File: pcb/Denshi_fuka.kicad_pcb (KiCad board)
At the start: 2 copper layers, 68.6 x 53.3 mm, 8 parts, among them J1 Power, J2 Digital/PWM, J3 Analog, J4 Digital/PWM

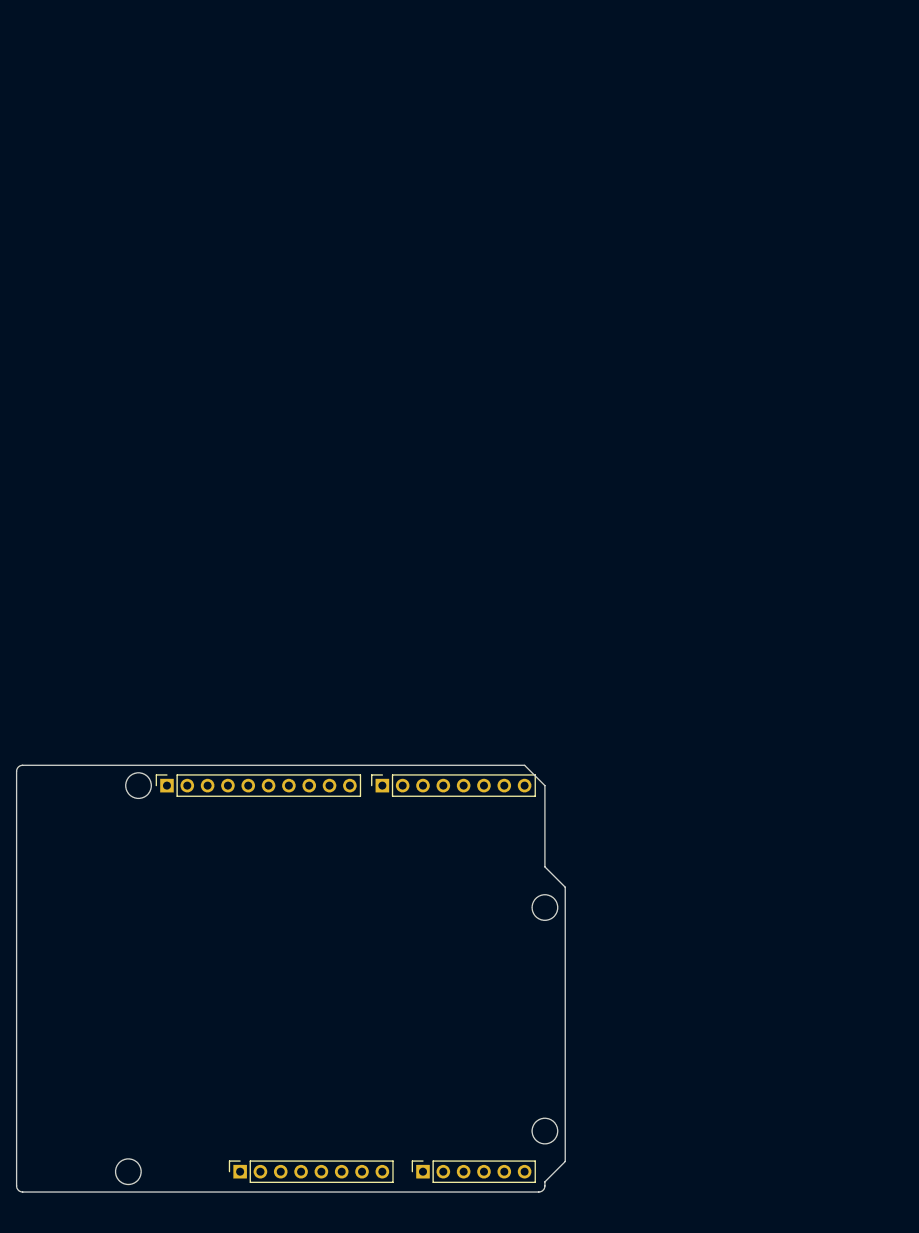
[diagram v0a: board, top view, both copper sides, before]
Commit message: Fuck
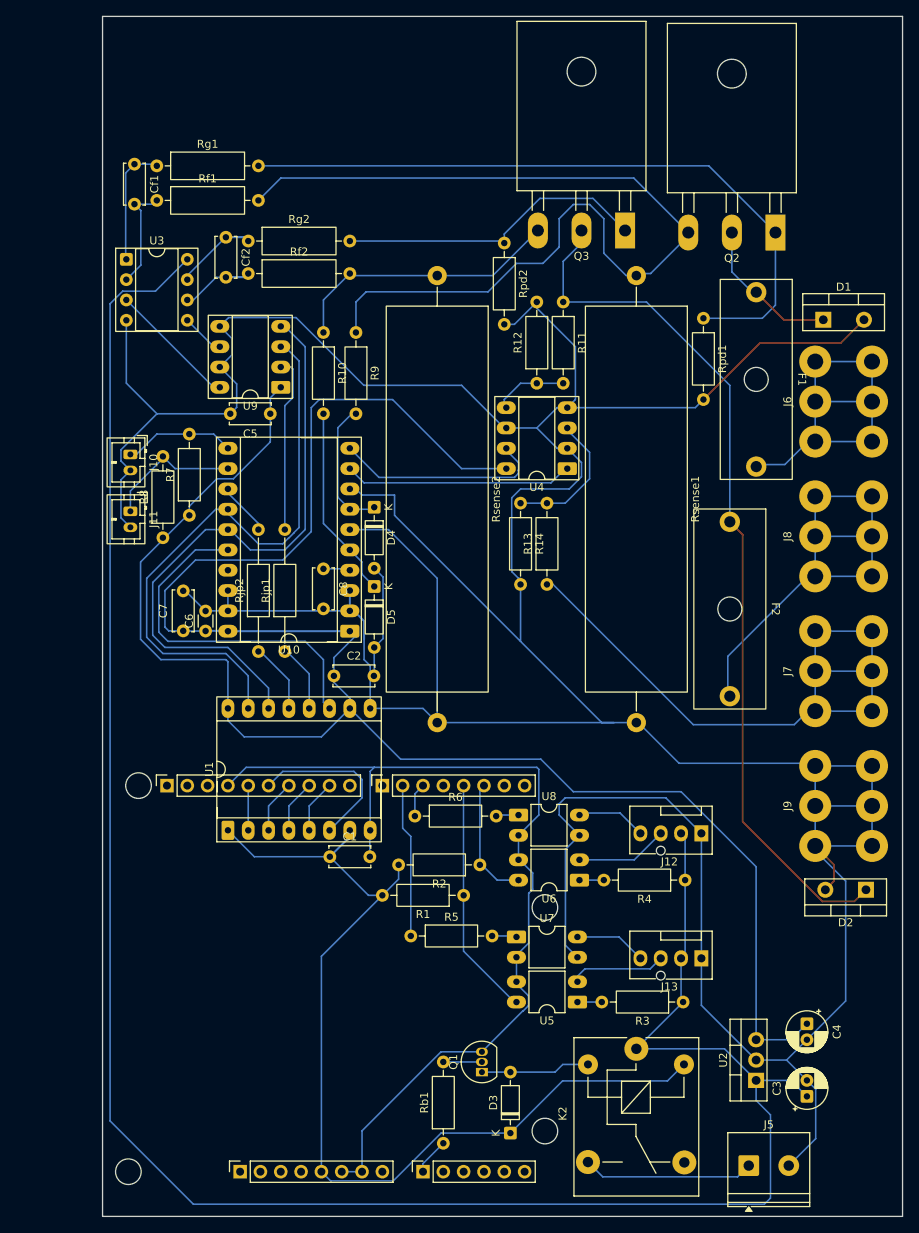
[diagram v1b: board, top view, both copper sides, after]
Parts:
- added C1: 0.1uF, Capacitor_THT:C_Disc_D5.0mm_W2.5mm_P5.00mm, F.Cu at (139.2, 58.1)
- added C2: 0.1uF, Capacitor_THT:C_Disc_D5.0mm_W2.5mm_P5.00mm, F.Cu at (139.7, 35.5)
- added C3: 10uF, Capacitor_THT:CP_Radial_D5.0mm_P2.00mm, F.Cu at (198.8, 88.0)
- added C4: 10uF, Capacitor_THT:CP_Radial_D5.0mm_P2.00mm, F.Cu at (198.8, 79.0)
- added C5: 0.1uF, Capacitor_THT:C_Disc_D5.0mm_W2.5mm_P5.00mm, F.Cu at (131.7, 2.72)
- added C6: 1uF, Capacitor_THT:C_Disc_D3.0mm_W1.6mm_P2.50mm, F.Cu at (123.6, 29.9)
- added C7: 0.1uF, Capacitor_THT:C_Disc_D5.0mm_W2.5mm_P5.00mm, F.Cu at (120.8, 29.9)
- added C8: 0.1uF, Capacitor_THT:C_Disc_D5.0mm_W2.5mm_P5.00mm, F.Cu at (138.4, 22.1)
- added Cf1: 0.1uF, Capacitor_THT:C_Disc_D5.0mm_W2.5mm_P5.00mm, F.Cu at (114.7, -28.5)
- added Cf2: 0.1uF, Capacitor_THT:C_Disc_D5.0mm_W2.5mm_P5.00mm, F.Cu at (126.2, -19.3)
- added D1: D, Package_TO_SOT_THT:TO-220-2_Vertical, F.Cu at (200.8, -9.03)
- added D2: D, Package_TO_SOT_THT:TO-220-2_Vertical, F.Cu at (206.2, 62.2)
- added D3: 1N4148, Diode_THT:D_DO-35_SOD27_P7.62mm_Horizontal, F.Cu at (161.7, 92.6)
- added D4: D_Zener_3V3, Diode_THT:D_DO-35_SOD27_P7.62mm_Horizontal, F.Cu at (144.7, 14.4)
- added D5: D_Zener_3V3, Diode_THT:D_DO-35_SOD27_P7.62mm_Horizontal, F.Cu at (144.7, 24.3)
- added F1: Fuse, MyParts:MF-563, F.Cu at (192.5, -1.58)
- added F2: Fuse, MyParts:MF-563, F.Cu at (189.2, 27.1)
- added J10: JST_PH2P, Connector_JST:JST_PH_B2B-PH-K_1x02_P2.00mm_Vertical, F.Cu at (114.2, 7.80)
- added J11: JST_PH2P, Connector_JST:JST_PH_B2B-PH-K_1x02_P2.00mm_Vertical, F.Cu at (114.2, 14.9)
- added J12: FAN_CONN1, Connector:FanPinHeader_1x04_P2.54mm_Vertical, F.Cu at (185.6, 55.2)
- added J13: FAN_CONN2, Connector:FanPinHeader_1x04_P2.54mm_Vertical, F.Cu at (185.6, 70.8)
- added J5: SCREW TERMINAL, TerminalBlock_Phoenix:TerminalBlock_Phoenix_PT-1,5-2-5.0-H_1x02_P5.00mm_Horizontal, F.Cu at (191.5, 96.7)
- added J6: SCREW TERMINAL, Aki-Parts:PCB-20, F.Cu at (203.4, 1.19)
- added J7: SCREW TERMINAL, Aki-Parts:PCB-20, F.Cu at (203.4, 34.9)
- added J8: SCREW TERMINAL, Aki-Parts:PCB-20, F.Cu at (203.4, 18.0)
- added J9: SCREW TERMINAL, Aki-Parts:PCB-20, F.Cu at (203.4, 51.7)
- added K2: SRD05VDCSLC, Relay_THT:Relay_SPDT_SANYOU_SRD_Series_Form_C, F.Cu at (177.5, 82.1)
- added Q1: 2SC1815, Package_TO_SOT_THT:TO-92_Inline, F.Cu at (158.2, 85.0)
- added Q2: 2SK3176, Package_TO_SOT_THT:TO-247-3_Horizontal_TabUp, F.Cu at (194.9, -19.9)
- added Q3: 2SK3176, Package_TO_SOT_THT:TO-247-3_Horizontal_TabUp, F.Cu at (176.1, -20.2)
- added R1: 10kΩ, Resistor_THT:R_Axial_DIN0207_L6.3mm_D2.5mm_P10.16mm_Horizontal, F.Cu at (155.9, 62.9)
- added R10: 1kΩ, Resistor_THT:R_Axial_DIN0207_L6.3mm_D2.5mm_P10.16mm_Horizontal, F.Cu at (138.4, -7.44)
- added R11: 1MΩ, Resistor_THT:R_Axial_DIN0207_L6.3mm_D2.5mm_P10.16mm_Horizontal, F.Cu at (168.3, -11.3)
- added R12: 10kΩ, Resistor_THT:R_Axial_DIN0207_L6.3mm_D2.5mm_P10.16mm_Horizontal, F.Cu at (165.0, -1.09)
- added R13: 100kΩ, Resistor_THT:R_Axial_DIN0207_L6.3mm_D2.5mm_P10.16mm_Horizontal, F.Cu at (166.3, 24.1)
- added R14: 22kΩ, Resistor_THT:R_Axial_DIN0207_L6.3mm_D2.5mm_P10.16mm_Horizontal, F.Cu at (163.0, 13.9)
- added R2: 10kΩ, Resistor_THT:R_Axial_DIN0207_L6.3mm_D2.5mm_P10.16mm_Horizontal, F.Cu at (157.9, 59.1)
- added R3: 1kΩ, Resistor_THT:R_Axial_DIN0207_L6.3mm_D2.5mm_P10.16mm_Horizontal, F.Cu at (183.3, 76.3)
- added R4: 1kΩ, Resistor_THT:R_Axial_DIN0207_L6.3mm_D2.5mm_P10.16mm_Horizontal, F.Cu at (183.6, 61.0)
- added R5: 220Ω, Resistor_THT:R_Axial_DIN0207_L6.3mm_D2.5mm_P10.16mm_Horizontal, F.Cu at (149.3, 68.0)
- added R6: 220Ω, Resistor_THT:R_Axial_DIN0207_L6.3mm_D2.5mm_P10.16mm_Horizontal, F.Cu at (149.8, 53.0)
- added R7: 10kΩ, Resistor_THT:R_Axial_DIN0207_L6.3mm_D2.5mm_P10.16mm_Horizontal, F.Cu at (121.6, 15.4)
- added R8: 10kΩ, Resistor_THT:R_Axial_DIN0207_L6.3mm_D2.5mm_P10.16mm_Horizontal, F.Cu at (118.3, 18.2)
- added R9: 1kΩ, Resistor_THT:R_Axial_DIN0207_L6.3mm_D2.5mm_P10.16mm_Horizontal, F.Cu at (142.4, -7.44)
- added Rb1: 1kΩ, Resistor_THT:R_Axial_DIN0207_L6.3mm_D2.5mm_P10.16mm_Horizontal, F.Cu at (153.3, 93.9)
- added Rf1: 1kΩ, Resistor_THT:R_Axial_DIN0309_L9.0mm_D3.2mm_P12.70mm_Horizontal, F.Cu at (117.5, -24.0)
- added Rf2: 1kΩ, Resistor_THT:R_Axial_DIN0309_L9.0mm_D3.2mm_P12.70mm_Horizontal, F.Cu at (129.0, -14.8)
- added Rg1: 1kΩ, Resistor_THT:R_Axial_DIN0309_L9.0mm_D3.2mm_P12.70mm_Horizontal, F.Cu at (117.5, -28.3)
- added Rg2: 1kΩ, Resistor_THT:R_Axial_DIN0309_L9.0mm_D3.2mm_P12.70mm_Horizontal, F.Cu at (129.0, -18.9)
- added Rjp1: 0Ω, Resistor_THT:R_Axial_DIN0207_L6.3mm_D2.5mm_P15.24mm_Horizontal, F.Cu at (133.5, 32.4)
- added Rjp2: 0Ω, Resistor_THT:R_Axial_DIN0207_L6.3mm_D2.5mm_P15.24mm_Horizontal, F.Cu at (130.2, 32.4)
- added Rpd1: 100kΩ, Resistor_THT:R_Axial_DIN0207_L6.3mm_D2.5mm_P10.16mm_Horizontal, F.Cu at (185.9, -9.22)
- added Rpd2: 100kΩ, Resistor_THT:R_Axial_DIN0207_L6.3mm_D2.5mm_P10.16mm_Horizontal, F.Cu at (161.0, -18.6)
- added Rsense1: 0.1Ω 10W, Resistor_THT:R_Axial_Power_L48.0mm_W12.5mm_P55.88mm, F.Cu at (177.5, -14.6)
- added Rsense2: 10Ω 10W, Resistor_THT:R_Axial_Power_L48.0mm_W12.5mm_P55.88mm, F.Cu at (152.6, -14.6)
- added U1: Si8651, MyParts:DIP-16_W15.24mm (600mil), F.Cu at (126.4, 54.8)
- added U10: MCP3564R, MyParts:DIP-20_W15.24mm_Socket_LongPads, F.Cu at (141.7, 29.9)
- added U2: LM2940T-3.3, Package_TO_SOT_THT:TO-220-3_Vertical, F.Cu at (192.4, 86.0)
- added U3: LM358, Package_DIP:DIP-8_W7.62mm_Socket, F.Cu at (113.7, -16.6)
- added U4: MCP6232, Package_DIP:DIP-8_W7.62mm_Socket_LongPads, F.Cu at (168.8, 9.58)
- added U5: PS817, Package_DIP:DIP-4_W7.62mm_LongPads, F.Cu at (170.1, 76.3)
- added U6: PS817, Package_DIP:DIP-4_W7.62mm_LongPads, F.Cu at (170.4, 61.0)
- added U7: PS817, Package_DIP:DIP-4_W7.62mm_LongPads, F.Cu at (162.5, 68.1)
- added U8: PS817, Package_DIP:DIP-4_W7.62mm_LongPads, F.Cu at (162.7, 52.9)
- added U9: MCP4822, Package_DIP:DIP-8_W7.62mm_Socket_LongPads, F.Cu at (133.0, -0.58)
- renumbered J3 to J2, J2 to J3
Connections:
- net /4 renamed /PD4
- net /7 renamed /PD7
- net /8 renamed /PB0
- net /A1 renamed /PC1
- net /A2 renamed /PC2
- net /A3 renamed /PC3
- net /RX/0 renamed /RXD/PD0
- net /SCL/A5 renamed /SCL/PC5
- net /SDA/A4 renamed /SDA/PC4
- net /TX/1 renamed /TXD/PD1
- net GND renamed GNDD
- net VCC renamed /Vin
- J1 pad 4: +3V3 -> unconnected-(J1-Pin_4-Pad4)
- J2 pad 1: /A0 -> /PC0
- J3 pad 5: /13 -> /SCK/PB5
- J3 pad 6: /12 -> /MISO/PB4
- J3 pad 7: /*11 -> /MOSI/PB3
- J3 pad 8: /*10 -> /PB2
- J3 pad 9: /*9 -> /PB1
- J4 pad 2: /*6 -> /PD6
- J4 pad 3: /*5 -> /PD5
- J4 pad 5: /*3 -> /PD3
- J4 pad 6: /2 -> /PD2
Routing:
- net GNDA: track 0.00 -> 567.3 mm
- net +3V3_A: track 0.00 -> 270.2 mm
- net +12V: track 0.00 -> 270.0 mm
- net +5V: track 0.00 -> 120.4 mm
- net GNDD: track 0.00 -> 120.1 mm
- net Net-(Q2-S): track 0.00 -> 119.0 mm
- net VDC2: track 0.00 -> 110.6 mm
- net Net-(Q2-G): track 0.00 -> 86.8 mm
- net VDC1_Sense: track 0.00 -> 82.4 mm
- net /SDI: track 0.00 -> 77.2 mm
- net /SCK: track 0.00 -> 75.6 mm
- net Net-(J8-Pin_1): track 0.00 -> 60.7 mm
- net Net-(J6-Pin_1): track 0.00 -> 49.9 mm
- net /SDO: track 0.00 -> 44.7 mm
- net Net-(Q3-G): track 0.00 -> 39.2 mm
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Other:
- board size 68.6 x 53.3 mm -> 100 x 150 mm
- board text removed: "ICSP"
